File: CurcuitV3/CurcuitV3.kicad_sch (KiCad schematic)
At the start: 94 parts, among them IC1 AS5600-ASOT, J1 Conn_01x02, J2 Conn_01x03, J3 Conn_01x07, J4 Conn_01x02, Q1 Q_NMOS_DGS, Q2 Q_NMOS_DGS, Q3 Q_NMOS_DGS, Q4 Q_NMOS_DGS, Q5 Q_NMOS_DGS, Q6 Q_NMOS_DGS, SW1 SW_Push, SW2 SW_Push, U1 DRV8300DPWR, U2 STM32F303K8Tx, U3 MCP9700x-ETT, U4 INA180A2, U5 LM66100DCK, U6 INA180A2, U7 AP7375-3.3, Y1 CSTNE16M0V530000R0

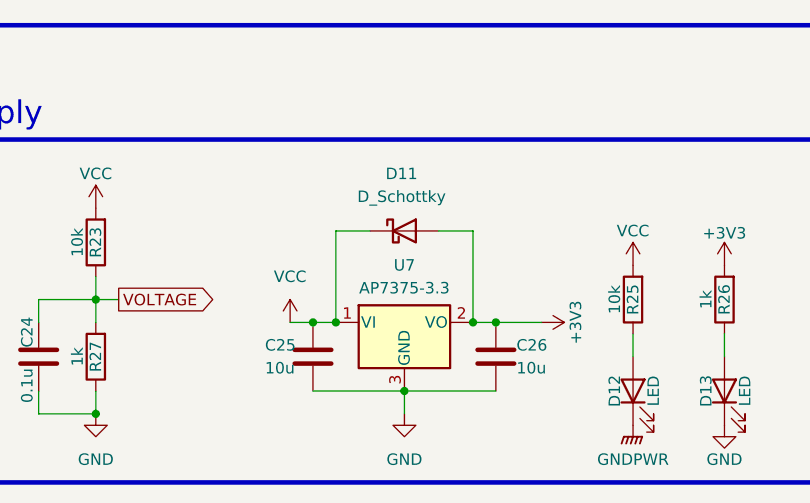
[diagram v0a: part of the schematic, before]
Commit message: シルク書いた
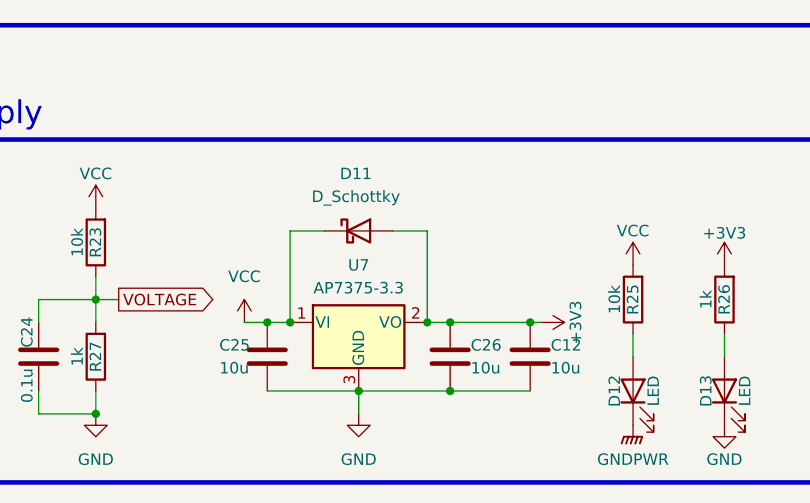
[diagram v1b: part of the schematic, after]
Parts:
- added C12: 10u, Capacitor_SMD:C_0805_2012Metric, symbol Device:C
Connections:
- net +3V3: now also C12.1
- net GND: now also C12.2
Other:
- moved on the sheet: C25, C26, D11, U7
